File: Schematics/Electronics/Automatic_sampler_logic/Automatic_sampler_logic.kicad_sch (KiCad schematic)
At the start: 14 parts, among them J1 MOT_X_SOCK, J2 MOT_Y_SOCK, J3 MOT_Z_SOCK, J4 Jack-DC, J5 FINAL_SOCK, J6 LCD_SOCK, J7 POWER_SOCK, J8 BUTTON_SOCK, U1 DRV8825, U2 DRV8825, U3 DRV8825, U4 Pico, U5 LM7805_TO220

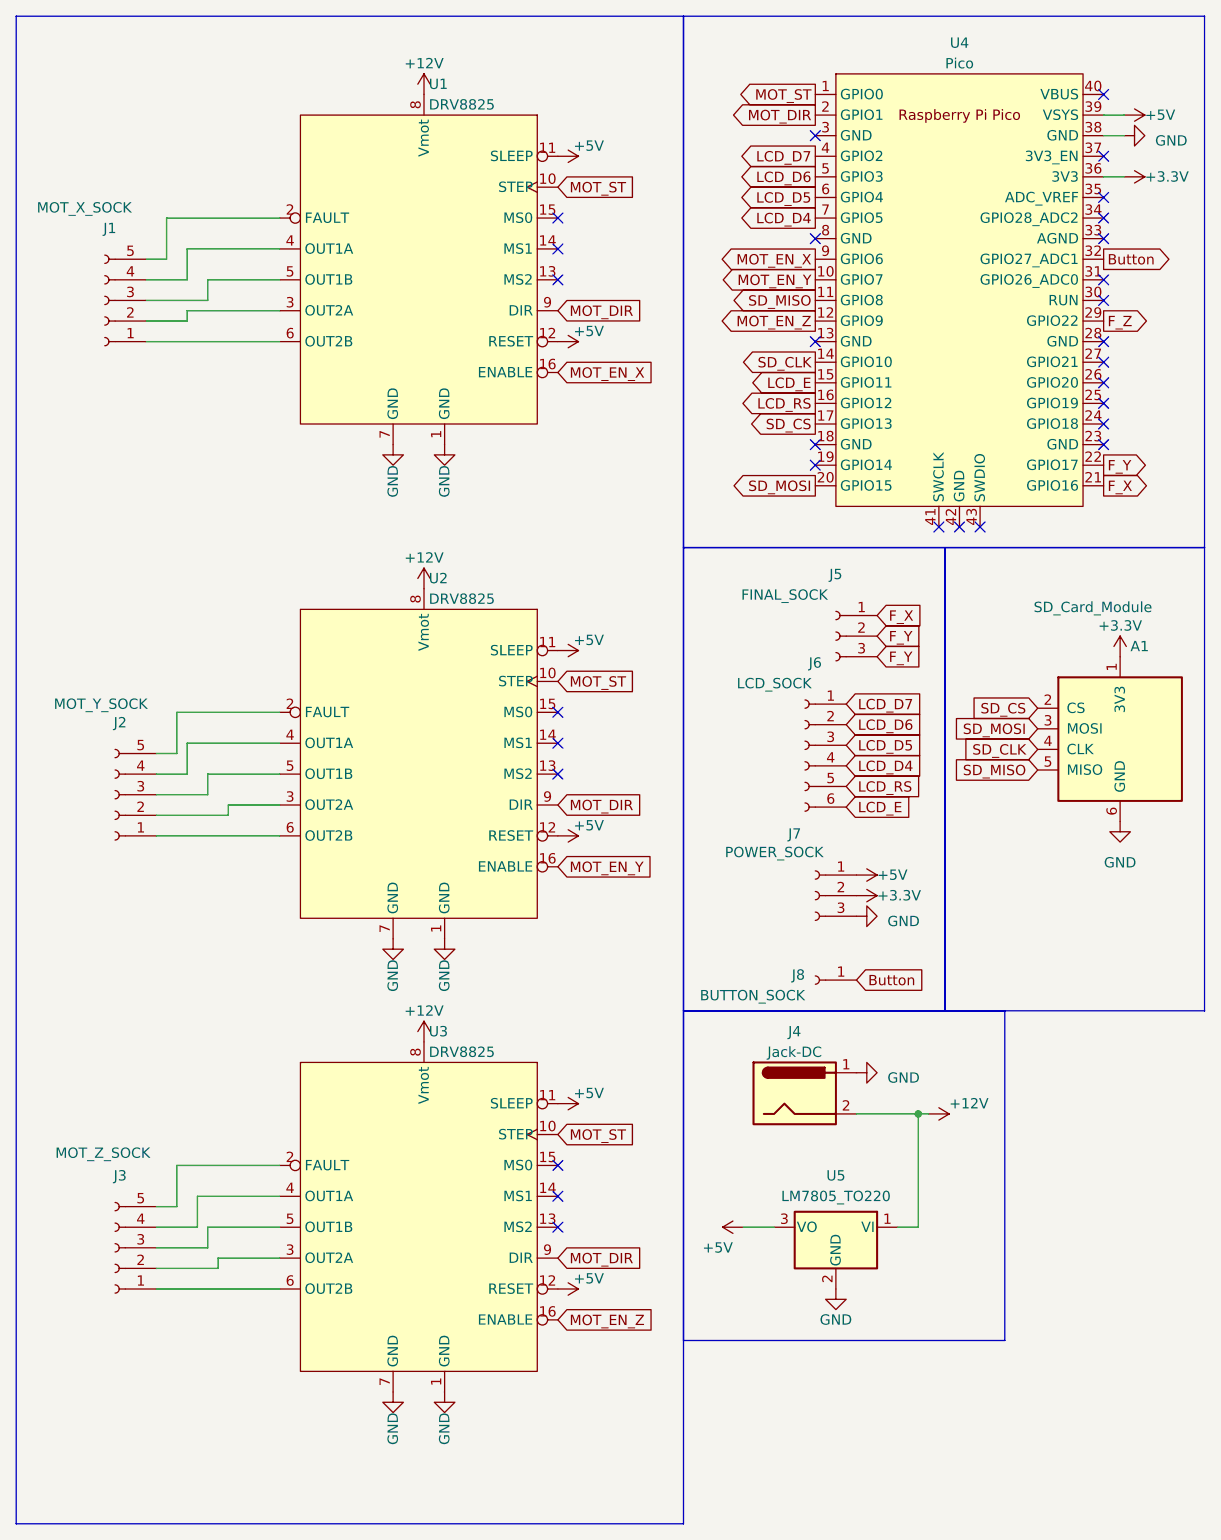
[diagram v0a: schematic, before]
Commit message: Changed schematics
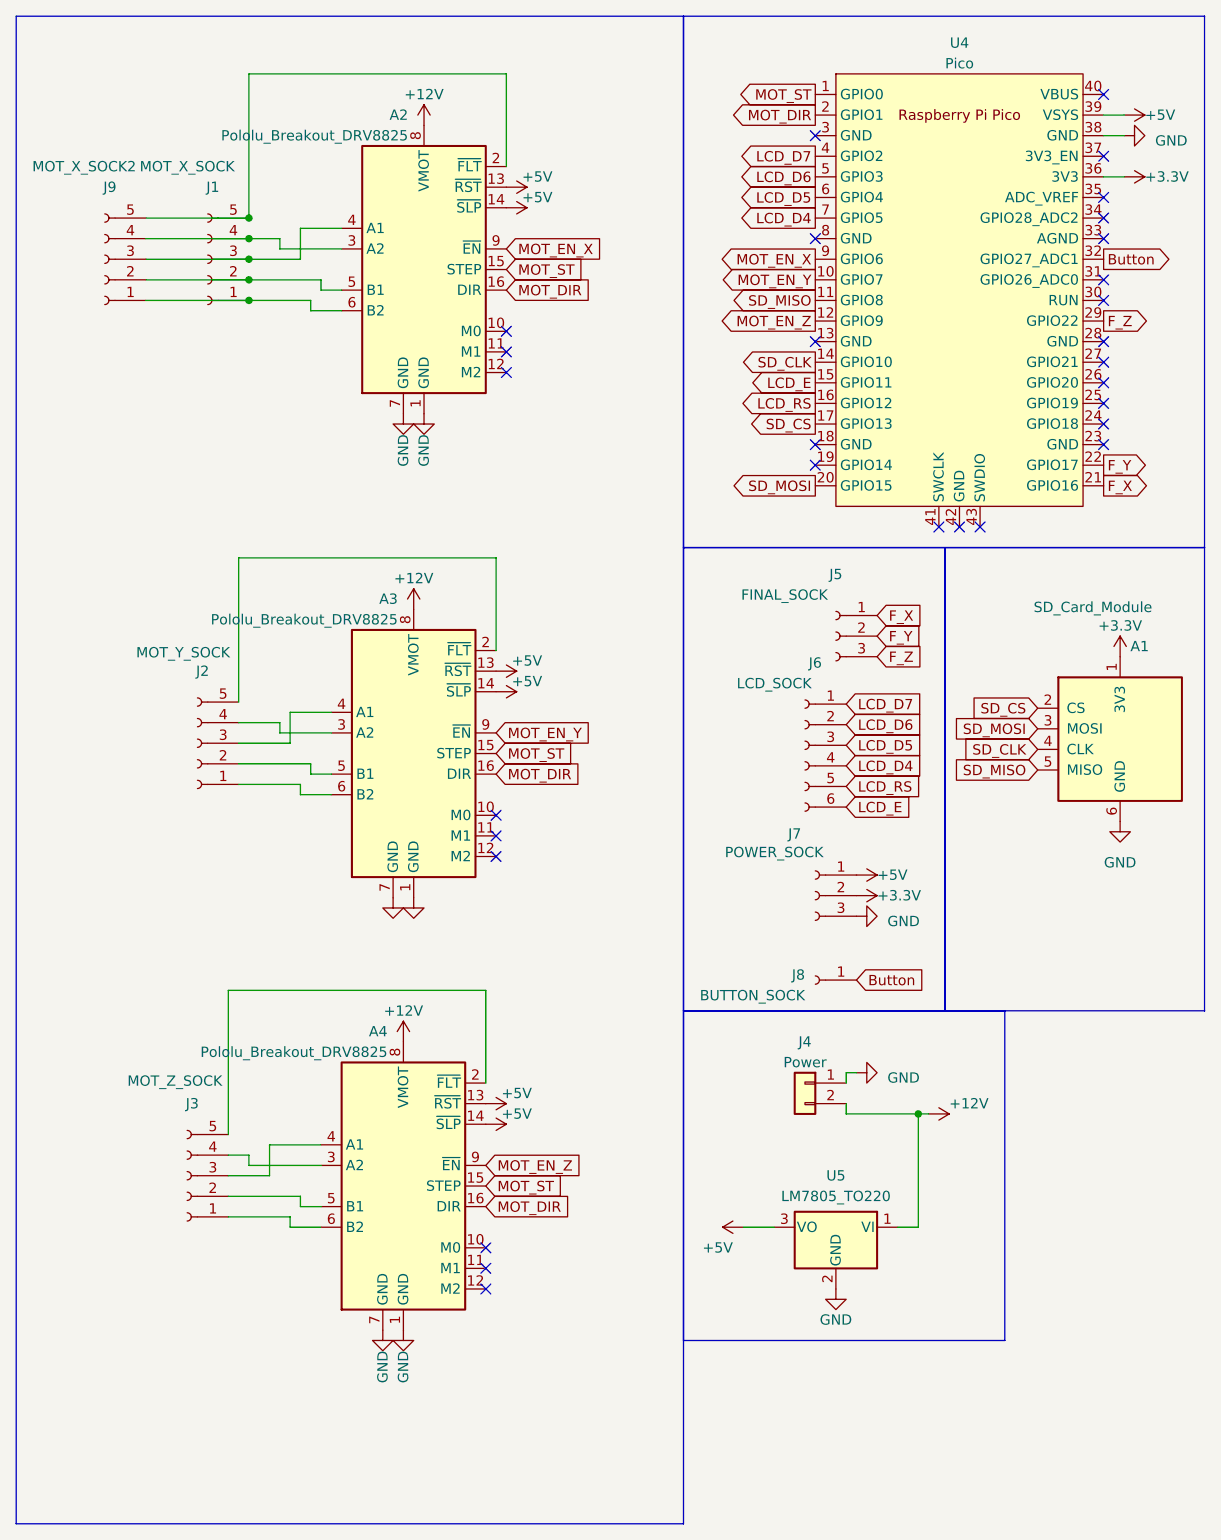
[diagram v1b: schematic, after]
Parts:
- removed J4: Jack-DC, Connector_BarrelJack:BarrelJack_Horizontal, symbol Connector:Jack-DC
- removed U1, U2, U3: DRV8825, symbol ATSS_Library:DRV8825
- added A2, A3, A4: Pololu_Breakout_DRV8825, Module:Pololu_Breakout-16_15.2x20.3mm, symbol Driver_Motor:Pololu_Breakout_DRV8825
- added J4: Power, Connector_PinSocket_2.54mm:PinSocket_1x02_P2.54mm_Vertical, symbol Connector_Generic:Conn_01x02
- added J9: MOT_X_SOCK2, Connector_PinSocket_2.54mm:PinSocket_1x05_P2.54mm_Vertical, symbol Connector:Conn_01x05_Socket
- J8: footprint (none) -> Connector_PinSocket_2.54mm:PinSocket_1x01_P2.54mm_Vertical
- U5: footprint (none) -> Package_TO_SOT_THT:TO-220-3_Vertical
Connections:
- net +12V: now also A2.8 (VMOT), A3.8 (VMOT), A4.8 (VMOT), J4.2 (Pin_2)
- net +5V: now also A2.13 (~{RST}), A2.14 (~{SLP}), A3.13 (~{RST}), A3.14 (~{SLP}), A4.13 (~{RST}), A4.14 (~{SLP})
- net F_Y: no longer J5.3 (Pin_3)
- net F_Z: now also J5.3 (Pin_3)
- net GND: now also A2.1 (GND), A2.7 (GND), A3.1 (GND), A3.7 (GND), A4.1 (GND), A4.7 (GND), J4.1 (Pin_1)
- net MOT_DIR: now also A2.16 (DIR), A3.16 (DIR), A4.16 (DIR)
- net MOT_EN_X: now also A2.9 (~{EN})
- net MOT_EN_Y: now also A3.9 (~{EN})
- net MOT_EN_Z: now also A4.9 (~{EN})
- net MOT_ST: now also A2.15 (STEP), A3.15 (STEP), A4.15 (STEP)
- net at J1.5 (Pin_5): now also A2.2 (~{FLT}), J9.5 (Pin_5)
- net at J1.2 (Pin_2): now also A2.5 (B1), J9.2 (Pin_2)
- net at J1.4 (Pin_4): now also A2.3 (A2), J9.4 (Pin_4)
- net at J1.3 (Pin_3): now also A2.4 (A1), J9.3 (Pin_3)
- net at J1.1 (Pin_1): now also A2.6 (B2), J9.1 (Pin_1)
- net at J2.1 (Pin_1): now also A3.6 (B2)
- net at J2.2 (Pin_2): now also A3.5 (B1)
- net at J2.3 (Pin_3): now also A3.4 (A1)
- net at J2.4 (Pin_4): now also A3.3 (A2)
- net at J2.5 (Pin_5): now also A3.2 (~{FLT})
- net at J3.5 (Pin_5): now also A4.2 (~{FLT})
- net at J3.2 (Pin_2): now also A4.5 (B1)
- net at J3.4 (Pin_4): now also A4.3 (A2)
- net at J3.3 (Pin_3): now also A4.4 (A1)
- net at J3.1 (Pin_1): now also A4.6 (B2)
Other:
- moved on the sheet: J1, J2, J3

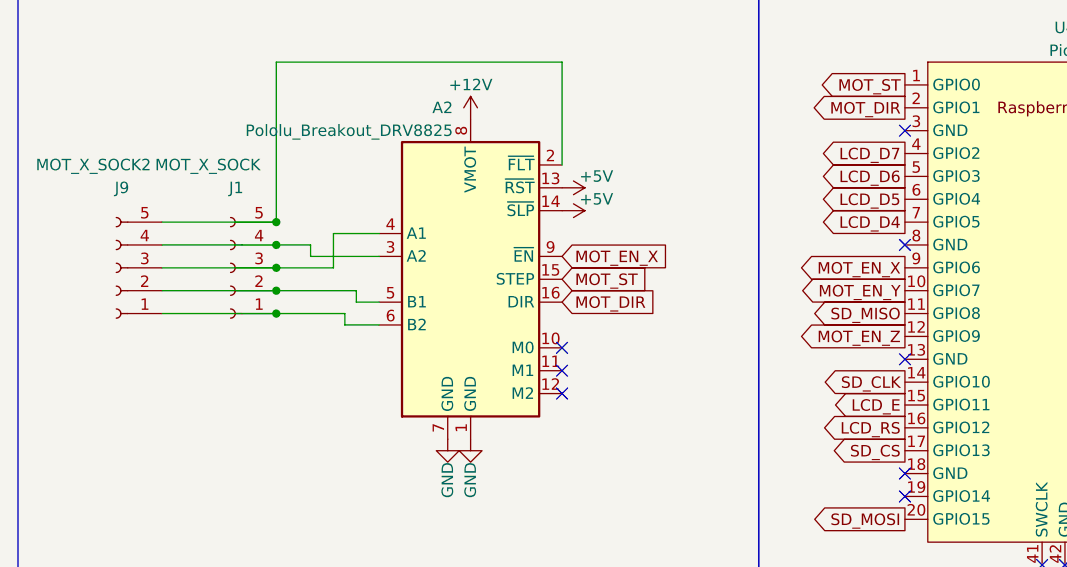
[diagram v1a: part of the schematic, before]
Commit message: Correcting errors
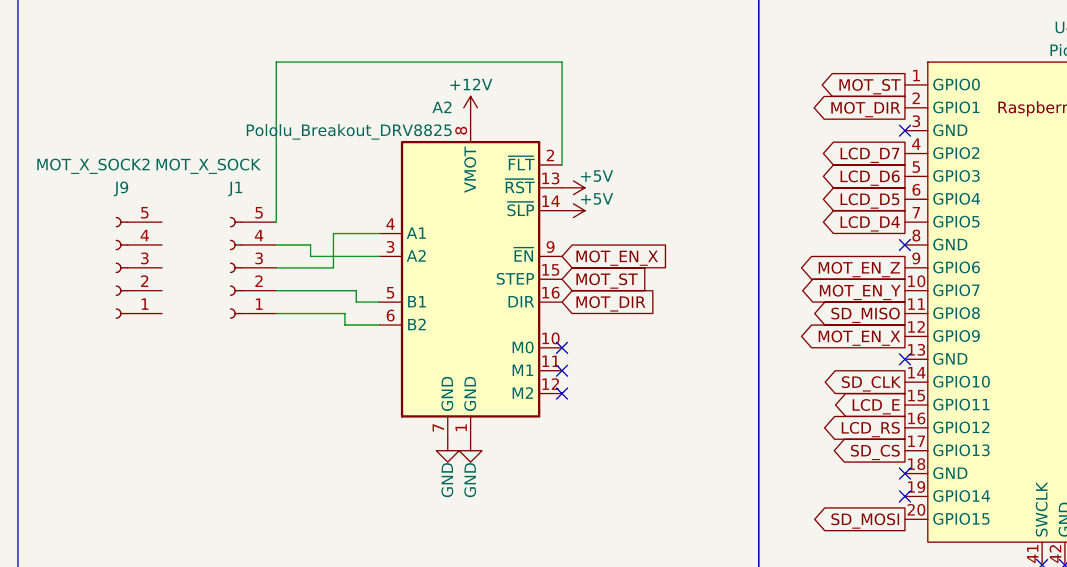
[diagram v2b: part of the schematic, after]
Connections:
- net MOT_EN_X: now also U4.12 (GPIO9); no longer U4.9 (GPIO6)
- net MOT_EN_Z: now also U4.9 (GPIO6); no longer U4.12 (GPIO9)
- net at A2.6 (B2), J1.1 (Pin_1): no longer J9.1 (Pin_1)
- net at A2.5 (B1), J1.2 (Pin_2): no longer J9.2 (Pin_2)
- net at A2.4 (A1), J1.3 (Pin_3): no longer J9.3 (Pin_3)
- net at A2.3 (A2), J1.4 (Pin_4): no longer J9.4 (Pin_4)
- net at A2.2 (~{FLT}), J1.5 (Pin_5): no longer J9.5 (Pin_5)
